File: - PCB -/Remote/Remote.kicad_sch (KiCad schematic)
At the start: 49 parts, among them J1 Conn_01x02_Pin, J2 Conn_01x02_Pin, J3 Conn_01x02_Pin, J4 AVR-ISP-6, J5 Conn_01x02_Pin, Q1 NMOS, SW1 SW_Push, SW2 SW_Push, SW3 SW_Push, SW4 SW_DIP_x05, U1 ATmega168PA-A, Y1 Crystal

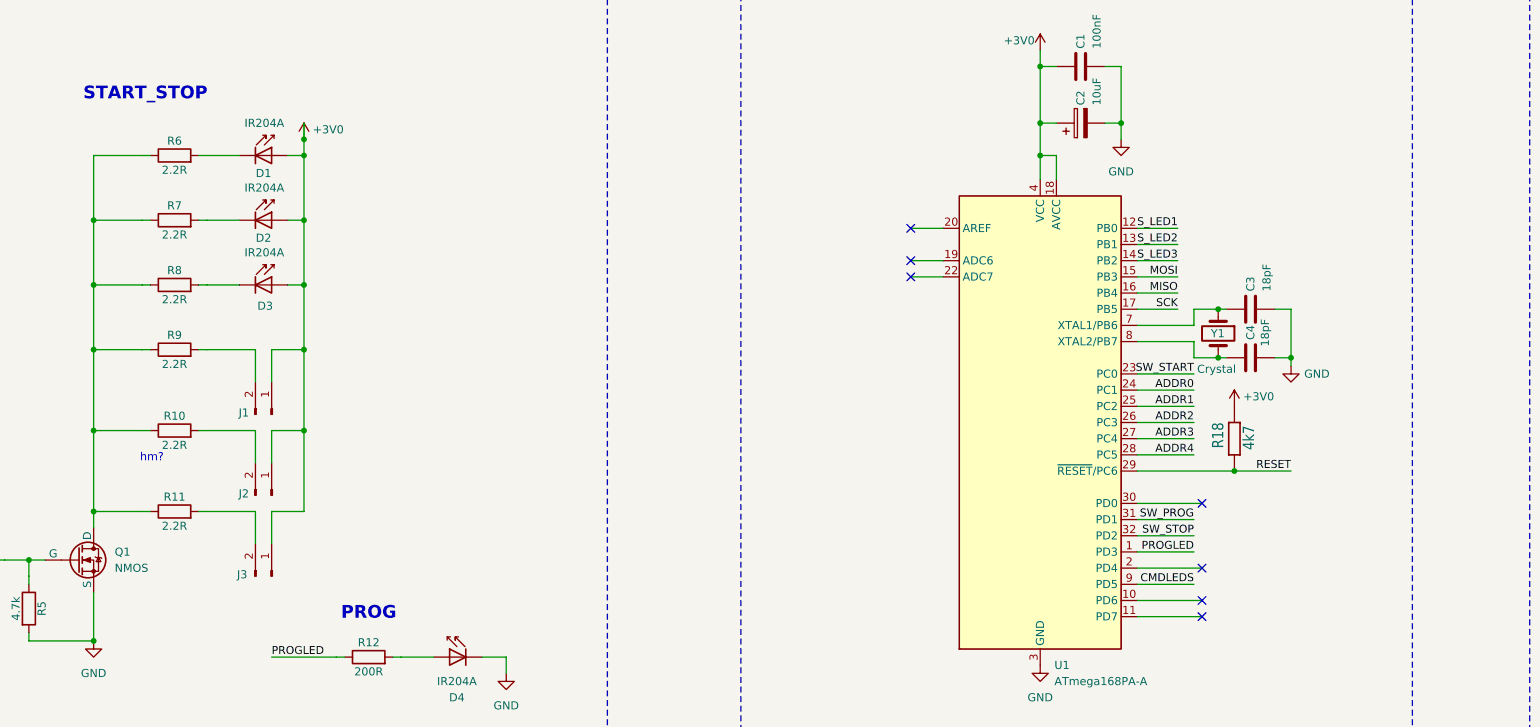
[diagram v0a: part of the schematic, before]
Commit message: Update Remote.kicad_sch
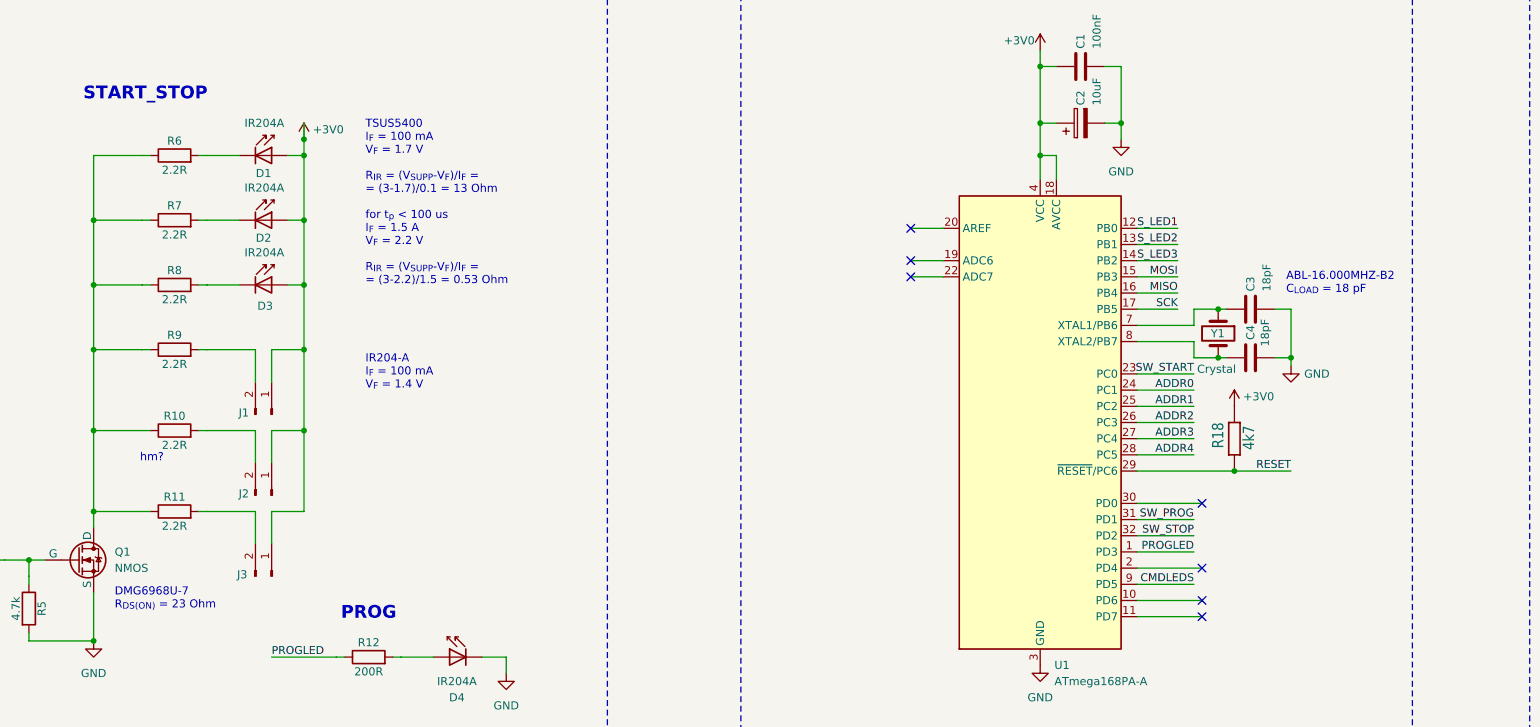
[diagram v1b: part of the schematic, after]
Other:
- note added: "ABL-16.000MHZ-B2 C_{LOAD} = 18 pF"
- note added: "DMG6968U-7 R_{DS(ON)} = 23 Ohm"
- note added: "IR204-A I_{F} = 100 mA V_{F} = 1.4 V"
- note added: "TSUS5400 I_{F} = 100 mA V_{F} = 1.7 V R_{IR} = (V_{SUPP}-V_{F})/I_{F} = = (3-1.7)/0.1 = 13 Ohm for t_{p} < 100 us I_{F} = 1.5 A V_{F} = 2.2 V R_{IR} = (V_{SUPP}-V_{F})/I_{F} = = (3-2.2)/1.5 = 0.53 Ohm"
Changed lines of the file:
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@@
+		)
+	)
+	(text "IR204-A\nI_{F} = 100 mA\nV_{F} = 1.4 V"
+		(exclude_from_sim no)
+		(at 118.872 89.662 0)
+		(effects
+			(font
+				(size 1.27 1.27)
+			)
+			(justify left top)
 		)
 	)
@@
 		)
 	)
+	(text "TSUS5400\nI_{F} = 100 mA\nV_{F} = 1.7 V\n\nR_{IR} = (V_{SUPP}-V_{F})/I_{F} =\n= (3-1.7)/0.1 = 13 Ohm\n\nfor t_{p} < 100 us\nI_{F} = 1.5 A\nV_{F} = 2.2 V\n\nR_{IR} = (V_{SUPP}-V_{F})/I_{F} =\n= (3-2.2)/1.5 = 0.53 Ohm\n"
+		(exclude_from_sim no)
+		(at 118.872 52.832 0)
+		(effects
+			(font
+				(size 1.27 1.27)
+			)
+			(justify left top)
+		)
+	)
 	(text "S_LEDS"
 		(exclude_from_sim no)
@@
 				(color 0 0 0 1)
 			)
+		)
+	)
+	(text "ABL-16.000MHZ-B2\nC_{LOAD} = 18 pF"
+		(exclude_from_sim no)
+		(at 263.398 76.708 0)
+		(effects
+			(font
+				(size 1.27 1.27)
+			)
+			(justify left top)
+			(href "https://cz.mouser.com/datasheet/2/3/ABL-1774766.pdf")
 		)
 	)
@@
 		)
 	)
+	(text "DMG6968U-7\nR_{DS(ON)} = 23 Ohm"
+		(exclude_from_sim no)
+		(at 79.502 126.238 0)
+		(effects
+			(font
+				(size 1.27 1.27)
+			)
+			(justify left top)
+		)
+	)
